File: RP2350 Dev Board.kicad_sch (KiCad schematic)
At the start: 48 parts, among them U2 SM03B-SRSS-TB(LF)(SN)(P), U4 W25Q128

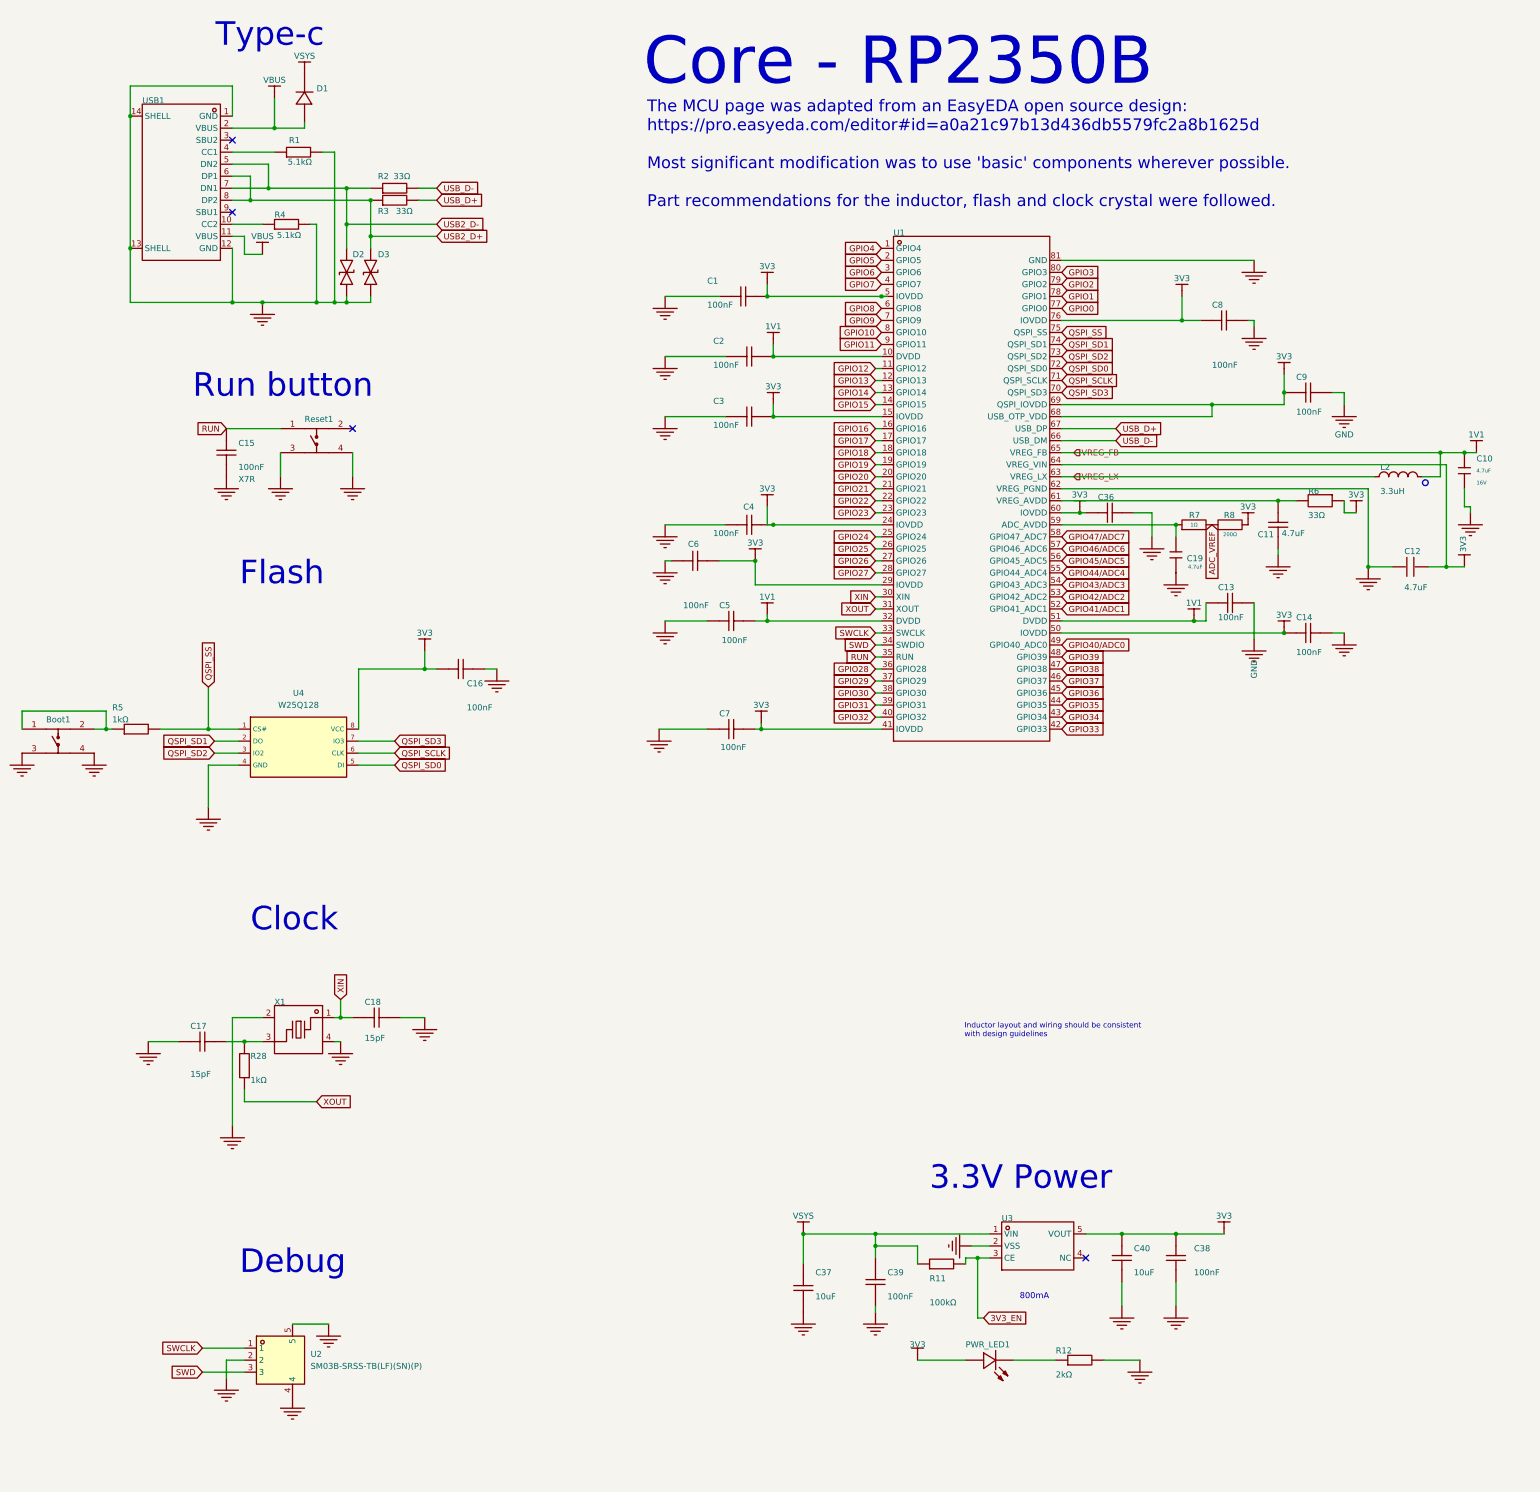
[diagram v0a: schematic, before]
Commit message: Re-did schematic
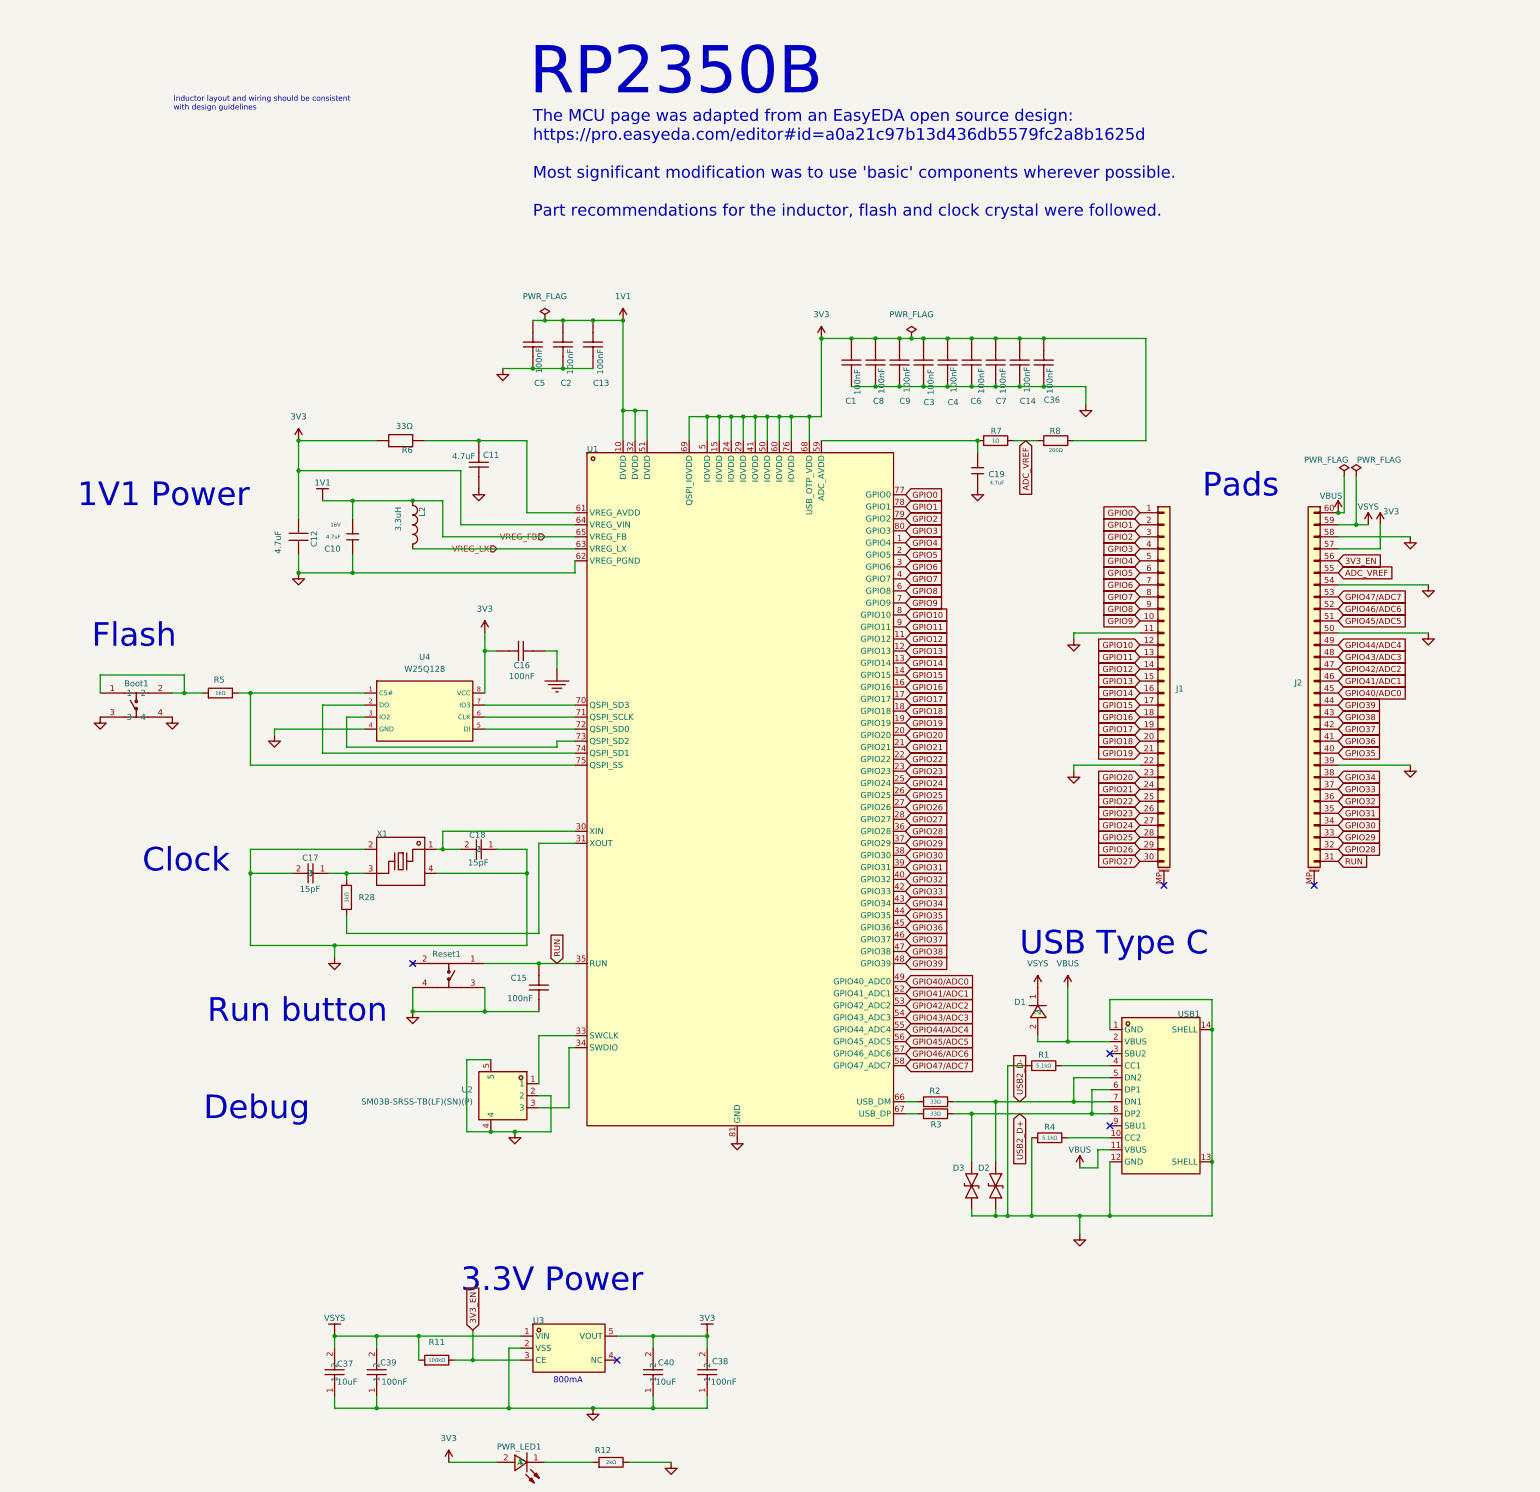
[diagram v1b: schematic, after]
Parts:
- removed R1, R4: 5.1kΩ, RP2350 Dev Board:, symbol ProPrj_RP2-easyedapro:0402WGJ0512TCE
- removed R11: 100kΩ, RP2350 Dev Board:R0402, symbol ProPrj_RP2-easyedapro:RC0402FR-07100KL
- removed R12: 2kΩ, RP2350 Dev Board:R0402, symbol ProPrj_RP2-easyedapro:0402WGF2001TCE
- removed R2, R3: 33Ω, RP2350 Dev Board:, symbol ProPrj_RP2-easyedapro:0402WGF270JTCE
- removed R28: 1kΩ, RP2350 Dev Board:, symbol ProPrj_RP2-easyedapro:0402WGF1001TCE
- removed R5: 1kΩ, RP2350 Dev Board:R0402, symbol ProPrj_RP2-easyedapro:0402WGJ0102TCE
- added J1, J2: Conn_01x30_MountingPin, symbol Connector_Generic_MountingPin:Conn_01x30_MountingPin
- added R1, R4: 5.1kΩ, PCM_JLCPCB:R_0402, symbol PCM_JLCPCB-Resistors:0402,5.1kΩ
- added R11: 100kΩ, PCM_JLCPCB:R_0402, symbol PCM_JLCPCB-Resistors:0402,100kΩ
- added R12: 2kΩ, PCM_JLCPCB:R_0402, symbol PCM_JLCPCB-Resistors:0402,2kΩ
- added R2, R3: 33Ω, PCM_JLCPCB:R_0402, symbol PCM_JLCPCB-Resistors:0402,33Ω
- added R28: 1kΩ, PCM_JLCPCB:R_0603, symbol PCM_JLCPCB-Resistors:0603,1kΩ
- added R5: 1kΩ, PCM_JLCPCB:R_0402, symbol PCM_JLCPCB-Resistors:0402,1kΩ
- Boot1: footprint RP2350 Dev Board:KEY-SMD_4P-L4.2-W3.2-P2.20-LS5.1-TL -> EasyEDA:KEY-SMD_4P-L4.2-W3.2-P2.20-LS5.1-TL; symbol ProPrj_RP2-easyedapro:K2-1808SN-A4SW -> EasyEDA:K2-1808SN-A4SW; LCSC Part (none) -> C92589
- C17, C18: footprint RP2350 Dev Board: -> EasyEDA:C0402; symbol ProPrj_RP2-easyedapro:GRM1555C1H100FA01D -> EasyEDA:0402CG150J500NT; LCSC Part (none) -> C1548
- C37, C40: footprint RP2350 Dev Board:C0402 -> EasyEDA:C0402; symbol ProPrj_RP2-easyedapro:GRM155R61A106ME44D -> EasyEDA:GRM155R61A106ME44D; LCSC Part (none) -> C77000
- C38, C39: footprint RP2350 Dev Board:C0402 -> EasyEDA:C0402; symbol ProPrj_RP2-easyedapro:GRM155R71H104KE14D -> EasyEDA:GRM155R71H104KE14D; LCSC Part (none) -> C77020
- D1: footprint RP2350 Dev Board:POWERDI-123_L2.8-W1.8-LS3.7-RD -> EasyEDA:POWERDI-123_L2.8-W1.8-LS3.7-RD; symbol ProPrj_RP2-easyedapro:DFLS130L-7 -> EasyEDA:DFLS130L-7; LCSC Part (none) -> C110493
- PWR_LED1: footprint RP2350 Dev Board:LED0402-RD -> EasyEDA:LED0402-RD; symbol ProPrj_RP2-easyedapro:FC-F1005HRK-620H5 -> EasyEDA:FC-F1005HRK-620H5; LCSC Part (none) -> C130719
- U1: footprint RP2350 Dev Board:QFN-80_L10.0-W10.0-P0.40-TL-EP3.4 -> EasyEDA:QFN-80_L10.0-W10.0-P0.40-TL-EP3.4; symbol ProPrj_RP2-easyedapro:RP2350B_C42415655 -> EasyEDA:RP2350B_C42415655; LCSC Part (none) -> C42415655
- U3: footprint RP2350 Dev Board:SOT-23-5_L3.0-W1.7-P0.95-LS2.8-BR -> EasyEDA:SOT-23-5_L3.0-W1.7-P0.95-LS2.8-BR; symbol ProPrj_RP2-easyedapro:ME6217C33M5G -> EasyEDA:ME6217C33M5G; LCSC Part (none) -> C427602
- USB1: footprint RP2350 Dev Board:USB-C-SMD_TYPE-C-6PIN-2MD-073 -> EasyEDA:USB-C-SMD_TYPE-C-6PIN-2MD-073; symbol ProPrj_RP2-easyedapro:TYPE-C 16PIN 2MD(073) -> EasyEDA:TYPE-C16PIN2MD(073); LCSC (none) -> C2765186; LCSC Part (none) -> C2765186
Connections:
- net 1V1: now also C10.2, C13.2, L2.1; no longer C10.1, C13.1, L2.2
- net 3V3: now also C12.2, C14.2, C36.2, C8.2, C9.2, J2.57 (Pin_57); no longer C12.1, C14.1, C36.1, C8.1, C9.1
- net 3V3_EN: now also J2.56 (Pin_56), R11.2
- net ADC_VREF: now also J2.55 (Pin_55)
- net GND: now also C10.1, C11.1, C12.1, C13.1, C14.1, C36.1, C8.1, C9.1, J1.11 (Pin_11), J1.22 (Pin_22), J2.39 (Pin_39), J2.50 (Pin_50), J2.54 (Pin_54), J2.58 (Pin_58), R1.1, R12.2, R4.1; no longer C10.2, C11.2, C12.2, C13.2, C14.2, C36.2, C8.2, C9.2
- net GPIO0: now also J1.1 (Pin_1)
- net GPIO1: now also J1.2 (Pin_2)
- net GPIO10: now also J1.12 (Pin_12)
- net GPIO11: now also J1.13 (Pin_13)
- net GPIO12: now also J1.14 (Pin_14)
- net GPIO13: now also J1.15 (Pin_15)
- net GPIO14: now also J1.16 (Pin_16)
- net GPIO15: now also J1.17 (Pin_17)
- net GPIO16: now also J1.18 (Pin_18)
- net GPIO17: now also J1.19 (Pin_19)
- net GPIO18: now also J1.20 (Pin_20)
- net GPIO19: now also J1.21 (Pin_21)
- net GPIO2: now also J1.3 (Pin_3)
- net GPIO20: now also J1.23 (Pin_23)
- net GPIO21: now also J1.24 (Pin_24)
- net GPIO22: now also J1.25 (Pin_25)
- net GPIO23: now also J1.26 (Pin_26)
- net GPIO24: now also J1.27 (Pin_27)
- net GPIO25: now also J1.28 (Pin_28)
- net GPIO26: now also J1.29 (Pin_29)
- net GPIO27: now also J1.30 (Pin_30)
- net GPIO28: now also J2.32 (Pin_32)
- net GPIO29: now also J2.33 (Pin_33)
- net GPIO3: now also J1.4 (Pin_4)
- net GPIO30: now also J2.34 (Pin_34)
- net GPIO31: now also J2.35 (Pin_35)
- net GPIO32: now also J2.36 (Pin_36)
- net GPIO33: now also J2.37 (Pin_37)
- net GPIO34: now also J2.38 (Pin_38)
- net GPIO35: now also J2.40 (Pin_40)
- net GPIO36: now also J2.41 (Pin_41)
- net GPIO37: now also J2.42 (Pin_42)
- net GPIO38: now also J2.43 (Pin_43)
- net GPIO39: now also J2.44 (Pin_44)
- net GPIO4: now also J1.5 (Pin_5)
- net GPIO40/ADC0: now also J2.45 (Pin_45)
- net GPIO41/ADC1: now also J2.46 (Pin_46)
- net GPIO42/ADC2: now also J2.47 (Pin_47)
- net GPIO43/ADC3: now also J2.48 (Pin_48)
- net GPIO44/ADC4: now also J2.49 (Pin_49)
- net GPIO45/ADC5: now also J2.51 (Pin_51)
- net GPIO46/ADC6: now also J2.52 (Pin_52)
- net GPIO47/ADC7: now also J2.53 (Pin_53)
- net GPIO5: now also J1.6 (Pin_6)
- net GPIO6: now also J1.7 (Pin_7)
- net GPIO7: now also J1.8 (Pin_8)
- net GPIO8: now also J1.9 (Pin_9)
- net GPIO9: now also J1.10 (Pin_10)
- net RUN: now also J2.31 (Pin_31)
- net USB2_D+: now also R3.2
- net USB2_D-: now also R2.2
- net VBUS: now also J2.60 (Pin_60)
- net VREG_LX: now also L2.2; no longer L2.1
- net VSYS: now also J2.59 (Pin_59), R11.1
- net at Boot1.1, Boot1.2: now also R5.1
- net at USB1.10 (CC2): now also R4.2
- net at USB1.4 (CC1): now also R1.2
- net at R6.2, U1.61 (VREG_AVDD): now also C11.2; no longer C11.1
- net at C17.1, X1.3: now also R28.1
- net at PWR_LED1.1 (K): now also R12.1
- net QSPI_SCLK: no longer names the net of U1.71 (QSPI_SCLK), U4.6 (CLK)
- net QSPI_SD0: no longer names the net of U1.72 (QSPI_SD0), U4.5 (DI)
- net QSPI_SD1: no longer names the net of U1.74 (QSPI_SD1), U4.2 (DO)
- net QSPI_SD2: no longer names the net of U1.73 (QSPI_SD2), U4.3 (IO2)
- net QSPI_SD3: no longer names the net of U1.70 (QSPI_SD3), U4.7 (IO3)
- net QSPI_SS: no longer names the net of U1.75 (QSPI_SS), U4.1 (CS#)
- net QSPI_SS: now also R5.2
- net SWCLK: no longer names the net of U1.33 (SWCLK), U2.1
- net SWD: no longer names the net of U1.34 (SWDIO), U2.3
- net USB_D+: no longer names the net of U1.67 (USB_DP)
- net USB_D+: now also R3.1
- net USB_D-: no longer names the net of U1.66 (USB_DM)
- net USB_D-: now also R2.1
- net XIN: no longer names the net of C18.2, U1.30 (XIN), X1.1
- net XOUT: no longer names the net of U1.31 (XOUT)
- net XOUT: now also R28.2
- no-connect marks 4 -> 6
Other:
- note added: "1V1 Power"
- note added: "Pads"
- note added: "RP2350B"
- note added: "USB Type C"
- note removed: "Core - RP2350B"
- note removed: "Type-c"
- moved on the sheet: Boot1, C1, C10, C11, C12, C13, C14, C15, C16, C17, C18, C19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
